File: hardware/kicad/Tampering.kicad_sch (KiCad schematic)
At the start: 4 parts

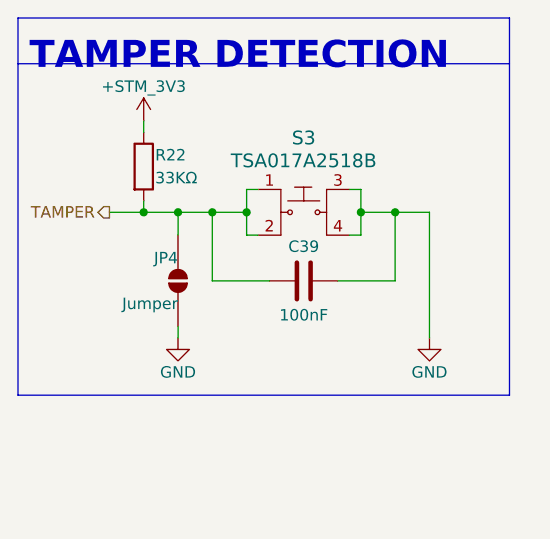
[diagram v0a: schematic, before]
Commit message: Final hardware cleanup push (hopefully)
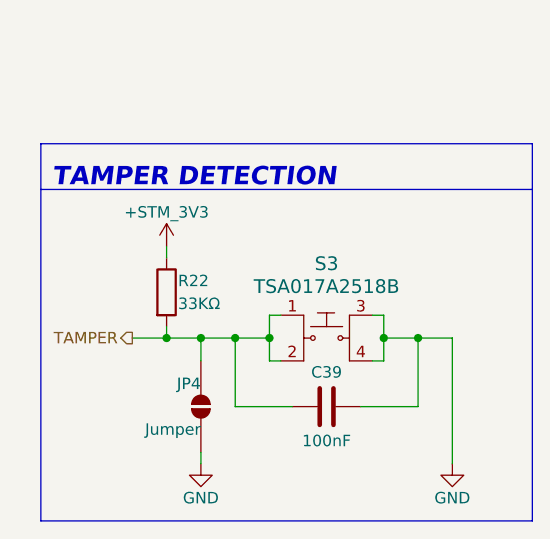
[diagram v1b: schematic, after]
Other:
- company: (none) -> Done By :- Arudhran
- title: (none) -> Cryptographic Tactical Node
- moved on the sheet: C39, JP4, R22, S3
